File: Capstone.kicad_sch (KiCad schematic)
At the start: 4 parts, among them J2 Conn_01x08_Socket, U1 XIAO-ESP32-S3-DIP, U11 SN74HC161DR, U3 74LS151

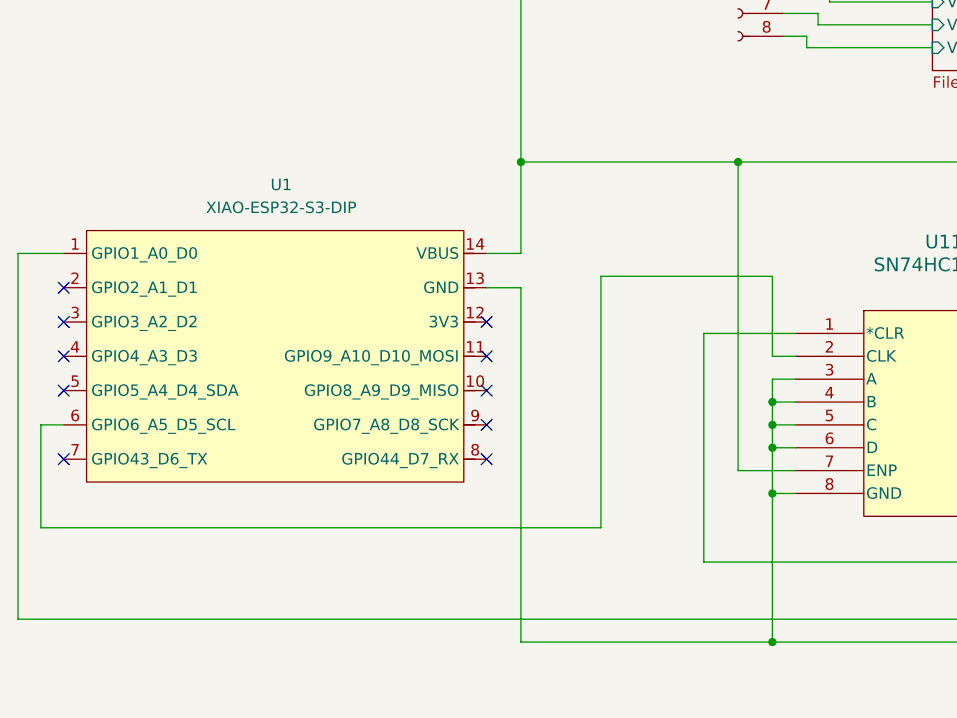
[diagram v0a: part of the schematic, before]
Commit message: Update Root
Working on simulations
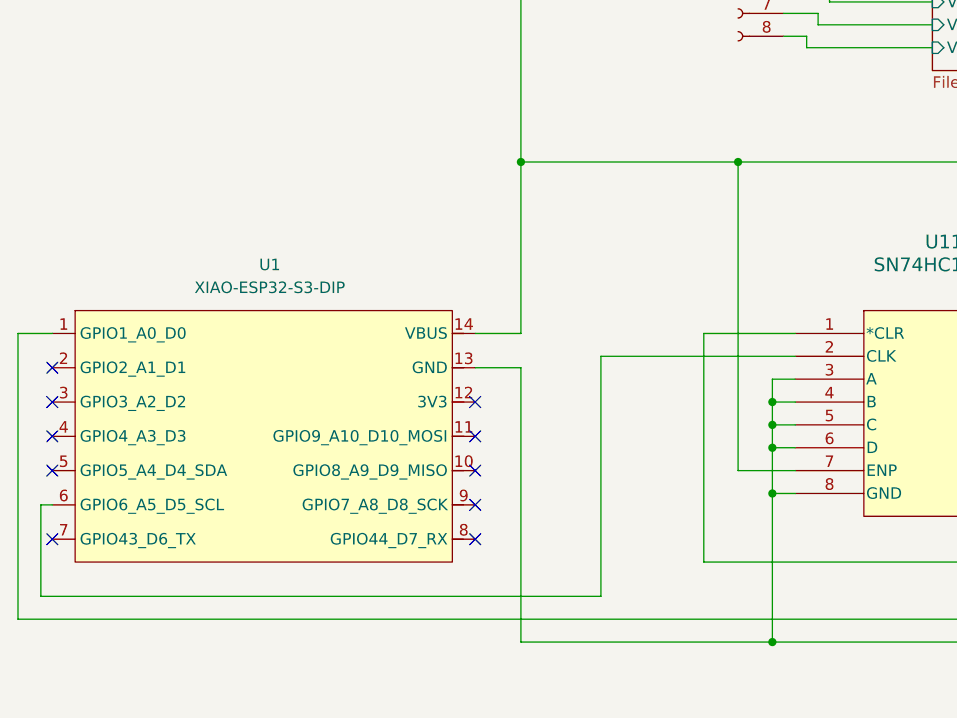
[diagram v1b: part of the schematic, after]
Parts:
- U1: footprint Seeed_Studio_XIAO_Series:XIAO-ESP32-S3-DIP -> CapstoneFootprints:XIAO-ESP32-S3-DIP
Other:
- moved on the sheet: U1
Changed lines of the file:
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@@
 	)
 	(no_connect
-		(at 30.48 78.74)
+		(at 29.21 87.63)
 	)
 	(no_connect
-		(at 30.48 74.93)
+		(at 29.21 83.82)
 	)
 	(no_connect
-		(at 77.47 93.98)
+		(at 76.2 102.87)
 	)
 	(no_connect
@@
 	)
 	(no_connect
-		(at 30.48 86.36)
+		(at 29.21 95.25)
 	)
 	(no_connect
-		(at 77.47 86.36)
+		(at 76.2 95.25)
 	)
 	(no_connect
-		(at 30.48 82.55)
+		(at 29.21 91.44)
 	)
 	(no_connect
-		(at 77.47 90.17)
+		(at 76.2 99.06)
 	)
 	(no_connect
-		(at 77.47 78.74)
+		(at 76.2 87.63)
 	)
 	(no_connect
@@
 	)
 	(no_connect
-		(at 77.47 82.55)
+		(at 76.2 91.44)
 	)
 	(no_connect
-		(at 30.48 93.98)
-	)
-	(wire
-		(pts
-			(xy 77.47 74.93) (xy 81.28 74.93)
+		(at 29.21 102.87)
+	)
+	(wire
+		(pts
+			(xy 76.2 83.82) (xy 81.28 83.82)
 		)
 		(stroke
@@
 	(wire
 		(pts
-			(xy 81.28 74.93) (xy 81.28 114.3)
+			(xy 81.28 83.82) (xy 81.28 114.3)
 		)
 		(stroke
@@
 	(wire
 		(pts
-			(xy 90.17 73.66) (xy 109.22 73.66)
+			(xy 90.17 82.55) (xy 111.76 82.55)
 		)
 		(stroke
@@
 	(wire
 		(pts
-			(xy 90.17 101.6) (xy 90.17 73.66)
+			(xy 90.17 109.22) (xy 90.17 82.55)
 		)
 		(stroke
@@
 	(wire
 		(pts
-			(xy 30.48 90.17) (xy 27.94 90.17)
-		)
-		(stroke
-			(width 0)
-			(type default)
-		)
-	)
-	(wire
-		(pts
-			(xy 27.94 90.17) (xy 27.94 101.6)
+			(xy 29.21 99.06) (xy 27.94 99.06)
+		)
+		(stroke
+			(width 0)
+			(type default)
+		)
+	)
+	(wire
+		(pts
+			(xy 27.94 99.06) (xy 27.94 109.22)
 		)
 		(stroke
@@
 	(wire
 		(pts
-			(xy 25.4 71.12) (xy 30.48 71.12)
-		)
-		(stroke
-			(width 0)
-			(type default)
-		)
-	)
-	(wire
-		(pts
-			(xy 25.4 111.76) (xy 25.4 71.12)
+			(xy 25.4 80.01) (xy 29.21 80.01)
+		)
+		(stroke
+			(width 0)
+			(type default)
+		)
+	)
+	(wire
+		(pts
+			(xy 25.4 111.76) (xy 25.4 80.01)
 		)
 		(stroke
@@
 	(wire
 		(pts
-			(xy 81.28 71.12) (xy 81.28 60.96)
+			(xy 81.28 80.01) (xy 81.28 60.96)
 		)
 		(stroke
@@
 	(wire
 		(pts
-			(xy 27.94 101.6) (xy 90.17 101.6)
+			(xy 27.94 109.22) (xy 90.17 109.22)
 		)
 		(stroke
@@
 	(wire
 		(pts
-			(xy 109.22 82.55) (xy 109.22 73.66)
-		)
-		(stroke
-			(width 0)
-			(type default)
-		)
-	)
-	(wire
-		(pts
 			(xy 149.86 43.18) (xy 149.86 40.64)
 		)
@@
 	(wire
 		(pts
-			(xy 111.76 82.55) (xy 109.22 82.55)
-		)
-		(stroke
-			(width 0)
-			(type default)
-		)
-	)
-	(wire
-		(pts
 			(xy 115.57 43.18) (xy 127 43.18)
 		)
@@
 	(wire
 		(pts
-			(xy 77.47 71.12) (xy 81.28 71.12)
+			(xy 76.2 80.01) (xy 81.28 80.01)
 		)
 		(stroke
@@
 	(symbol
 		(lib_id "Seeed_Studio_XIAO_Series:XIAO-ESP32-S3-DIP")
-		(at 33.02 66.04 0)
+		(at 31.75 74.93 0)
 		(unit 1)
-		(exclude_from_sim no)
+		(exclude_from_sim yes)
 		(in_bom yes)
 		(on_board yes)
@@
 		(fields_autoplaced yes)
 		(property "Reference" "U1"
-			(at 54.6481 63.5 0)
+			(at 53.3781 72.39 0)
 			(effects
 				(font
@@
 		)
 		(property "Value" "XIAO-ESP32-S3-DIP"
-			(at 54.6481 66.04 0)
-			(effects
-				(font
-					(size 1.27 1.27)
-				)
-			)
-		)
-		(property "Footprint" "Seeed_Studio_XIAO_Series:XIAO-ESP32-S3-DIP"
-			(at 50.038 97.79 0)
+			(at 53.3781 74.93 0)
+			(effects
+				(font
+					(size 1.27 1.27)
+				)
+			)
+		)
+		(property "Footprint" "CapstoneFootprints:XIAO-ESP32-S3-DIP"
+			(at 48.768 106.68 0)
 			(effects
 				(font
@@
 		)
 		(property "Datasheet" ""
-			(at 33.02 66.04 0)
+			(at 31.75 74.93 0)
 			(effects
 				(font
@@
 		)
 		(property "Description" ""
-			(at 33.02 66.04 0)
+			(at 31.75 74.93 0)
 			(effects
 				(font
@@
 			(at 111.76 80.01 0)
 			(effects
+				(font
+					(size 1.27 1.27)
+				)
+				(hide yes)
+			)
+		)
+		(property "Sim.Library" ".\\"
+			(at 111.76 80.01 0)
+			(effects
